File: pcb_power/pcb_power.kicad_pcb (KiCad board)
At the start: 2 copper layers, 38 x 28.7 mm, 34 parts, among them J1 Pwr_jmp, J2 CPU_jmp, J3 Serial Header, J4 Programming Header, SW1 SW_SPDT, SW2 SW_SPST, SW3 SW_SPST, SW4 SW_SPST, U1 RP402N331F, U2 LoRa-E5, U3 IN-S128TATRGB

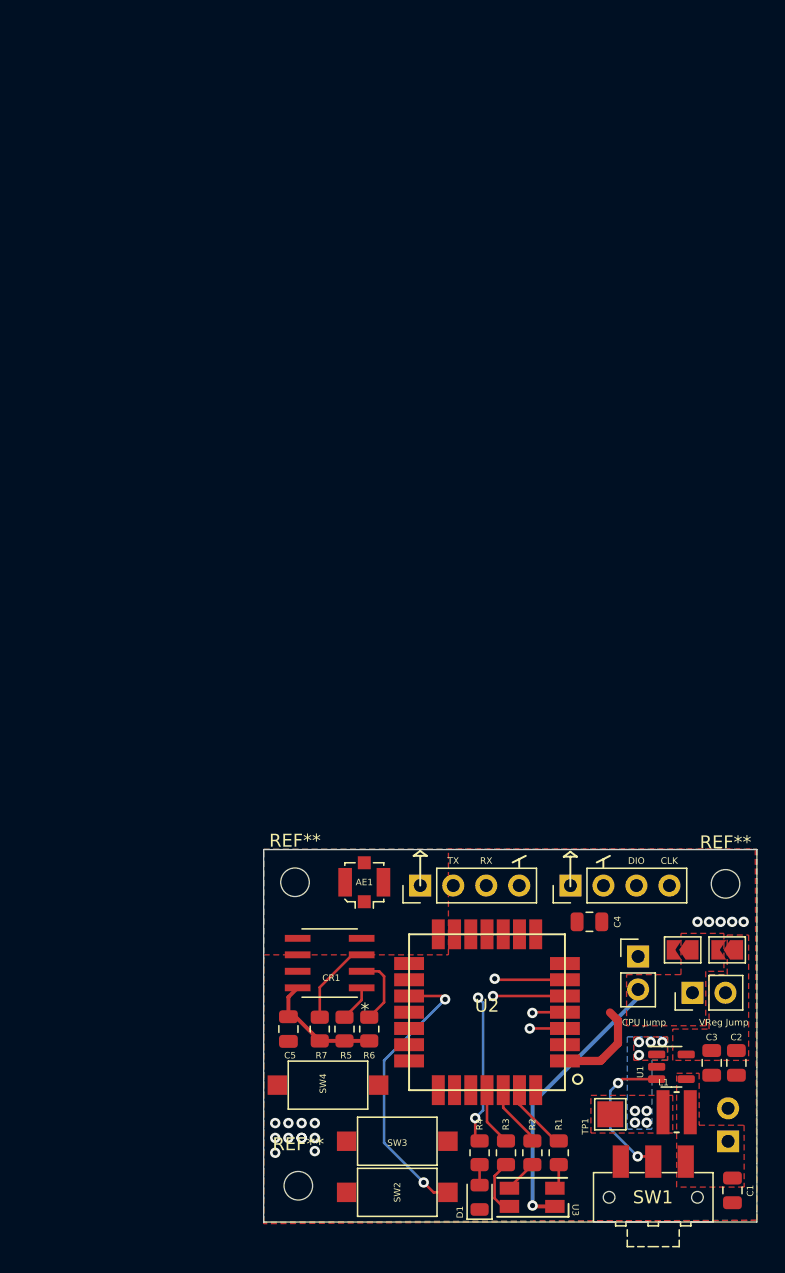
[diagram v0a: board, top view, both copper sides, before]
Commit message: DRC Fixes, etc
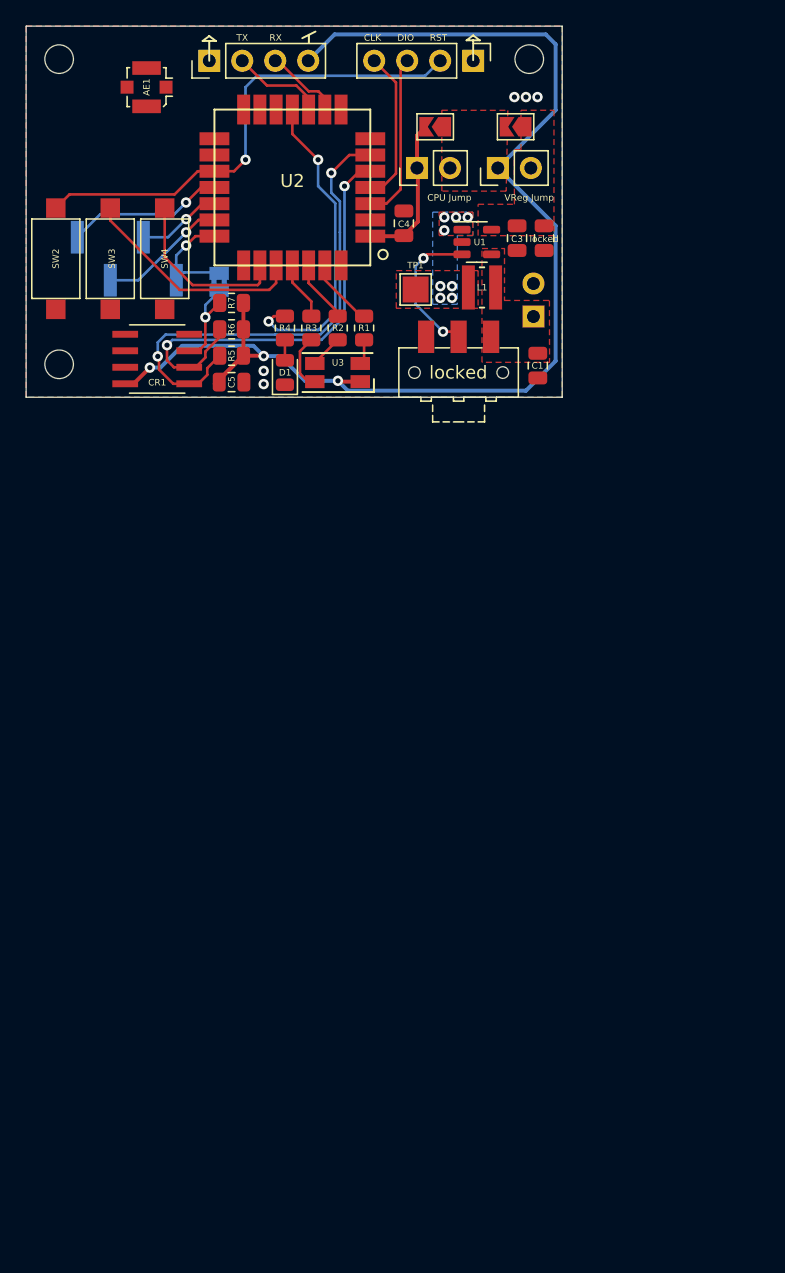
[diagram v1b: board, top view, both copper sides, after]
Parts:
- added J5: Pins Header, Connector_PinHeader_2.54mm:PinHeader_1x04_P2.54mm_Vertical_SMD_Pin1Left, B.Cu at (131.6, 40.1)
- added JP3: Pwr_jmp, Jumper:SolderJumper-2_P1.3mm_Bridged2Bar_Pad1.0x1.5mm, B.Cu at (138.7, 41.9)
- locked: renamed from SW1; value SW_SPDT -> locked
- locked: renamed from C2; value 10u -> locked
- moved SW2 76.5 mm to (126.1, 40.1), turned to -90 degrees
- moved SW3 71.4 mm to (130.3, 40.1), turned to -90 degrees
- moved JP2 66.2 mm to (155.3, 30.0)
- moved REF** 65.9 mm to (126.4, 24.8)
- moved REF** 65.9 mm to (126.4, 48.3)
- moved J3 65.5 mm to (137.9, 24.9)
- moved JP1 65.4 mm to (161.5, 30.0)
- moved REF** 65.3 mm to (162.6, 24.8)
- moved C3 65.2 mm to (161.6, 38.5)
- moved J1 65.2 mm to (160.1, 33.1)
- moved L1 65.2 mm to (158.9, 42.3)
- moved TP1 65.2 mm to (153.8, 42.5)
- moved U1 65.2 mm to (158.5, 38.8)
- moved U3 65.2 mm to (150.7, 50.5)
- moved BT1 65.2 mm to (162.9, 44.6)
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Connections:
- J4 pad 2: +3V3 -> RST
- U2 pad 18: unconnected-(U2-Pad18) -> PA3
- U2 pad 19: unconnected-(U2-Pad19) -> PA2
- U2 pad 20: unconnected-(U2-Pad20) -> PB10
- U2 pad 21: unconnected-(U2-Pad21) -> PA9
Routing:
- net +3V3: track 31.2 -> 97.1 mm, vias 1 -> 3
- net PA15/SDA: track 8.25 -> 38.1 mm, vias 1 -> 2
- net PB15/SCL: track 11.1 -> 34.4 mm, vias 1 -> 2
- net BOOT/PB13: track 0.91 -> 17.5 mm
- net RST: track 22.4 -> 37.6 mm, vias 2 -> 1
- net PA0/BUTTON: track 0.00 -> 13.4 mm
- net LED_STATUS: track 11.6 -> 24.4 mm
- net PA3: track 0.00 -> 12.1 mm, vias 0 -> 1
- net PB10: track 0.00 -> 9.94 mm, vias 0 -> 1
- net SWDIO/PA13: track 3.44 -> 12.9 mm, vias 1 -> 0
- net SWCLK/PA14: track 2.53 -> 11.8 mm, vias 1 -> 0
- net PA9: track 0.00 -> 9.01 mm, vias 0 -> 1
- net TX/PB6: track 0.00 -> 8.10 mm
- net PA2: track 0.00 -> 6.59 mm, vias 0 -> 1
- net RX/PB7: track 0.00 -> 5.91 mm
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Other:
- board size 38 x 28.7 mm -> 41.3 x 28.6 mm
- board text added: "A3"
- board text added: "A9"
- board text added: "B10"
- board text added: "RST"
